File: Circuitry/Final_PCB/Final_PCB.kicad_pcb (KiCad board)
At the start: 2 copper layers, 28 parts

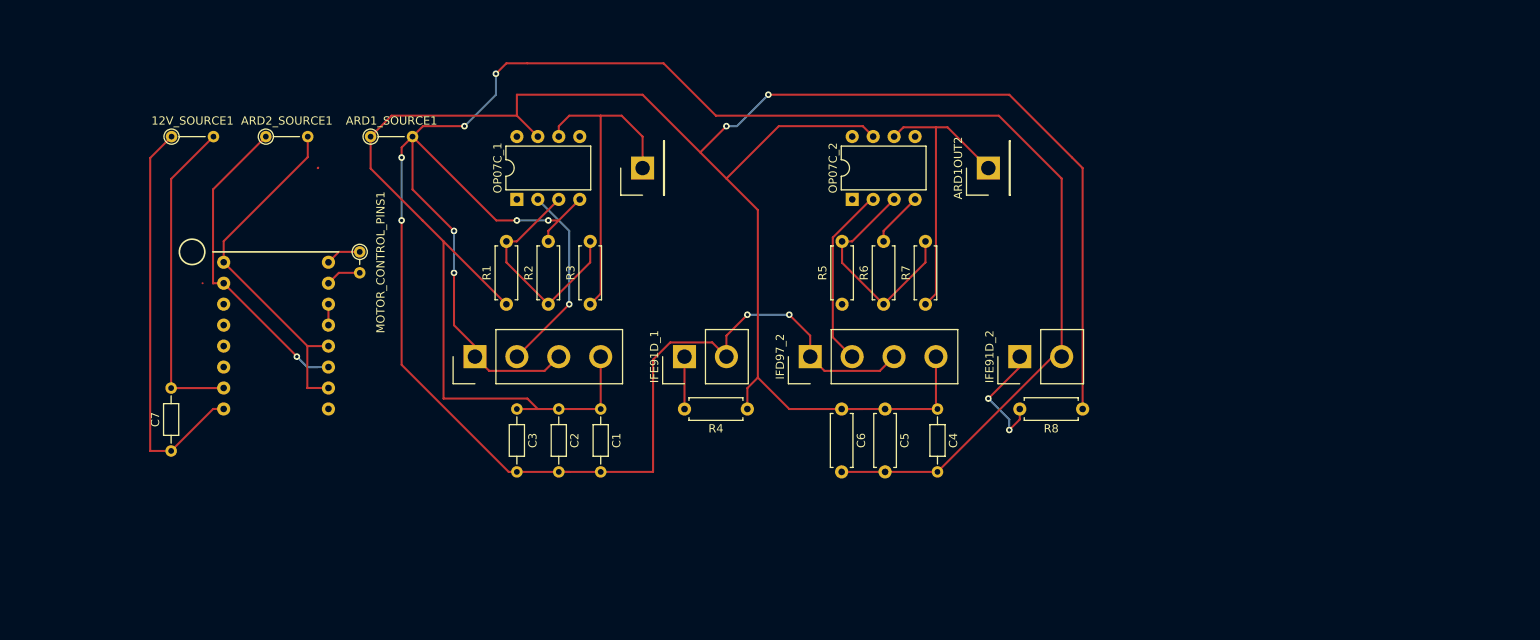
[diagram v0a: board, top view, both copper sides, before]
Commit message: PCB Finalized and updates to python program
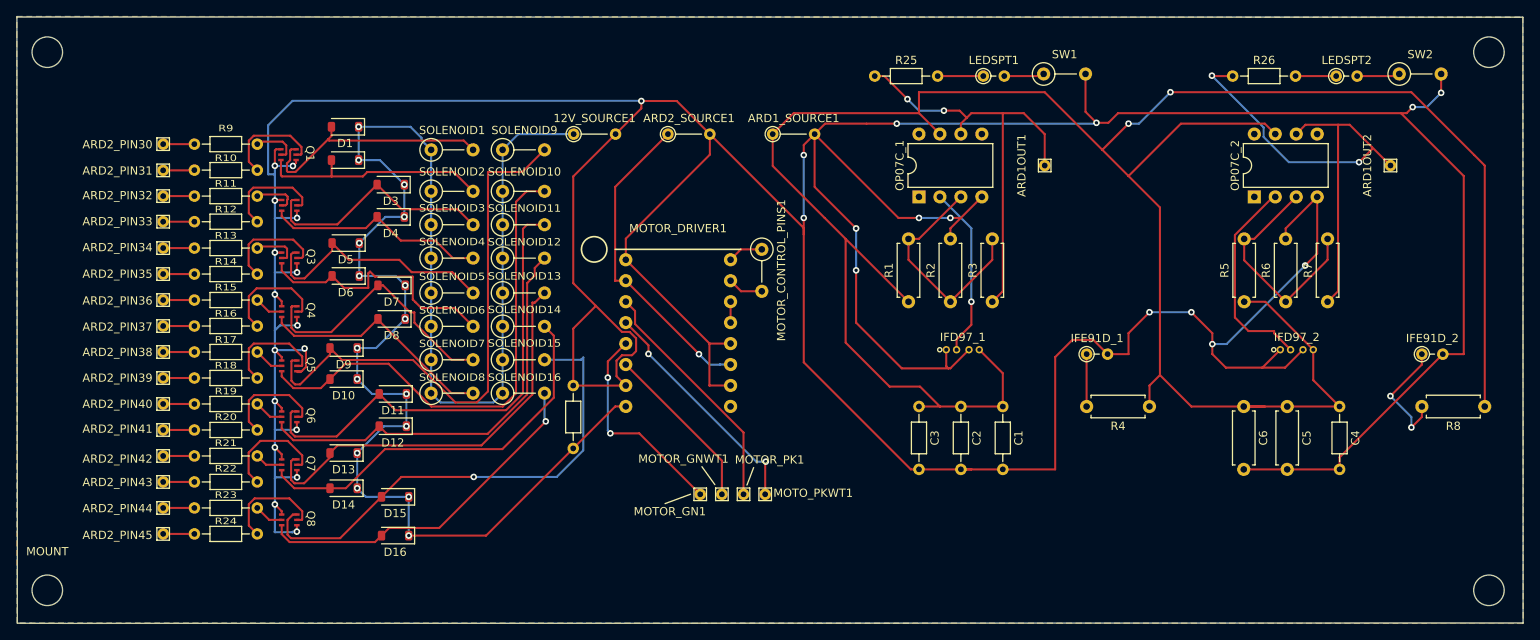
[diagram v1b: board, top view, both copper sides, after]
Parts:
- added ARD2_PIN30: Conn_01x01, Final_PCB_Footprint:ARD_OUT, F.Cu at (95.6, 82.2)
- added ARD2_PIN31: Conn_01x01, Final_PCB_Footprint:ARD_OUT, F.Cu at (95.6, 85.4)
- added ARD2_PIN32: Conn_01x01, Final_PCB_Footprint:ARD_OUT, F.Cu at (95.6, 88.5)
- added ARD2_PIN33: Conn_01x01, Final_PCB_Footprint:ARD_OUT, F.Cu at (95.6, 91.6)
- added ARD2_PIN34: Conn_01x01, Final_PCB_Footprint:ARD_OUT, F.Cu at (95.6, 94.8)
- added ARD2_PIN35: Conn_01x01, Final_PCB_Footprint:ARD_OUT, F.Cu at (95.6, 97.9)
- added ARD2_PIN36: Conn_01x01, Final_PCB_Footprint:ARD_OUT, F.Cu at (95.6, 101.1)
- added ARD2_PIN37: Conn_01x01, Final_PCB_Footprint:ARD_OUT, F.Cu at (95.6, 104.2)
- added ARD2_PIN38: Conn_01x01, Final_PCB_Footprint:ARD_OUT, F.Cu at (95.6, 107.4)
- added ARD2_PIN39: Conn_01x01, Final_PCB_Footprint:ARD_OUT, F.Cu at (95.6, 110.5)
- added ARD2_PIN40: Conn_01x01, Final_PCB_Footprint:ARD_OUT, F.Cu at (95.6, 113.7)
- added ARD2_PIN41: Conn_01x01, Final_PCB_Footprint:ARD_OUT, F.Cu at (95.6, 116.8)
- added ARD2_PIN42: Conn_01x01, Final_PCB_Footprint:ARD_OUT, F.Cu at (95.6, 120.0)
- added ARD2_PIN43: Conn_01x01, Final_PCB_Footprint:ARD_OUT, F.Cu at (95.6, 123.1)
- added ARD2_PIN44: Conn_01x01, Final_PCB_Footprint:ARD_OUT, F.Cu at (95.6, 126.3)
- added ARD2_PIN45: Conn_01x01, Final_PCB_Footprint:ARD_OUT, F.Cu at (95.6, 129.4)
- added D1: MBR0540, Diode_SMD:D_SOD-123, F.Cu at (117.6, 80.1)
- added D10: MBR0540, Diode_SMD:D_SOD-123, F.Cu at (117.4, 110.7)
- added D11: MBR0540, Diode_SMD:D_SOD-123, F.Cu at (123.4, 112.5)
- added D12: MBR0540, Diode_SMD:D_SOD-123, F.Cu at (123.4, 116.4)
- added D13: MBR0540, Diode_SMD:D_SOD-123, F.Cu at (117.4, 119.6)
- added D14: MBR0540, Diode_SMD:D_SOD-123, F.Cu at (117.4, 123.9)
- added D15: MBR0540, Diode_SMD:D_SOD-123, F.Cu at (123.7, 124.9)
- added D16: MBR0540, Diode_SMD:D_SOD-123, F.Cu at (123.7, 129.6)
- added D2: MBR0540, Diode_SMD:D_SOD-123, F.Cu at (117.6, 84.1)
- added D3: MBR0540, Diode_SMD:D_SOD-123, F.Cu at (123.1, 87.1)
- added D4: MBR0540, Diode_SMD:D_SOD-123, F.Cu at (123.1, 91.0)
- added D5: MBR0540, Diode_SMD:D_SOD-123, F.Cu at (117.7, 94.2)
- added D6: MBR0540, Diode_SMD:D_SOD-123, F.Cu at (117.7, 98.2)
- added D7: MBR0540, Diode_SMD:D_SOD-123, F.Cu at (123.2, 99.3)
- added D8: MBR0540, Diode_SMD:D_SOD-123, F.Cu at (123.2, 103.4)
- added D9: MBR0540, Diode_SMD:D_SOD-123, F.Cu at (117.4, 106.9)
- added LEDSPT1: Conn_01x02, Resistor_THT:R_Axial_DIN0204_L3.6mm_D1.6mm_P2.54mm_Vertical, F.Cu at (195.0, 73.9)
- added LEDSPT2: Conn_01x02, Resistor_THT:R_Axial_DIN0204_L3.6mm_D1.6mm_P2.54mm_Vertical, F.Cu at (237.7, 73.9)
- added MOTOR_GN1: Conn_01x01, Final_PCB_Footprint:ARD_OUT, F.Cu at (160.7, 124.6)
- added MOTOR_GNWT1: Conn_01x01, Final_PCB_Footprint:ARD_OUT, F.Cu at (163.3, 124.6)
- added MOTOR_PK1: Conn_01x01, Final_PCB_Footprint:ARD_OUT, F.Cu at (165.9, 124.6)
- added MOTO_PKWT1: Conn_01x01, Final_PCB_Footprint:ARD_OUT, F.Cu at (168.5, 124.6)
- added MOUNT: MountingHole_3.7mm, MountingHole:MountingHole_3.7mm, F.Cu at (81.5, 136.3)
- added Q1: Q_Dual_NMOS_S1G1D2S2G2D1, Final_PCB_Footprint:TSOP6_MOSFET, F.Cu at (110.7, 83.5)
- added Q2: Q_Dual_NMOS_S1G1D2S2G2D1, Final_PCB_Footprint:TSOP6_MOSFET, F.Cu at (110.8, 89.6)
- added Q3: Q_Dual_NMOS_S1G1D2S2G2D1, Final_PCB_Footprint:TSOP6_MOSFET, F.Cu at (110.8, 96.0)
- added Q4: Q_Dual_NMOS_S1G1D2S2G2D1, Final_PCB_Footprint:TSOP6_MOSFET, F.Cu at (110.8, 102.5)
- added Q5: Q_Dual_NMOS_S1G1D2S2G2D1, Final_PCB_Footprint:TSOP6_MOSFET, F.Cu at (110.8, 109.1)
- added Q6: Q_Dual_NMOS_S1G1D2S2G2D1, Final_PCB_Footprint:TSOP6_MOSFET, F.Cu at (110.8, 115.2)
- added Q7: Q_Dual_NMOS_S1G1D2S2G2D1, Final_PCB_Footprint:TSOP6_MOSFET, F.Cu at (110.8, 121.1)
- added Q8: Q_Dual_NMOS_S1G1D2S2G2D1, Final_PCB_Footprint:TSOP6_MOSFET, F.Cu at (110.8, 127.7)
- added R10: R, Resistor_THT:R_Axial_DIN0204_L3.6mm_D1.6mm_P7.62mm_Horizontal, F.Cu at (99.3, 85.3)
- added R11: R, Resistor_THT:R_Axial_DIN0204_L3.6mm_D1.6mm_P7.62mm_Horizontal, F.Cu at (99.3, 88.5)
- added R12: R, Resistor_THT:R_Axial_DIN0204_L3.6mm_D1.6mm_P7.62mm_Horizontal, F.Cu at (99.3, 91.6)
- added R13: R, Resistor_THT:R_Axial_DIN0204_L3.6mm_D1.6mm_P7.62mm_Horizontal, F.Cu at (99.3, 94.8)
- added R14: R, Resistor_THT:R_Axial_DIN0204_L3.6mm_D1.6mm_P7.62mm_Horizontal, F.Cu at (99.3, 97.9)
- added R15: R, Resistor_THT:R_Axial_DIN0204_L3.6mm_D1.6mm_P7.62mm_Horizontal, F.Cu at (99.3, 101.1)
- added R16: R, Resistor_THT:R_Axial_DIN0204_L3.6mm_D1.6mm_P7.62mm_Horizontal, F.Cu at (99.3, 104.2)
- added R17: R, Resistor_THT:R_Axial_DIN0204_L3.6mm_D1.6mm_P7.62mm_Horizontal, F.Cu at (99.3, 107.4)
- added R18: R, Resistor_THT:R_Axial_DIN0204_L3.6mm_D1.6mm_P7.62mm_Horizontal, F.Cu at (99.3, 110.5)
- added R19: R, Resistor_THT:R_Axial_DIN0204_L3.6mm_D1.6mm_P7.62mm_Horizontal, F.Cu at (99.3, 113.7)
- added R20: R, Resistor_THT:R_Axial_DIN0204_L3.6mm_D1.6mm_P7.62mm_Horizontal, F.Cu at (99.3, 116.8)
- added R21: R, Resistor_THT:R_Axial_DIN0204_L3.6mm_D1.6mm_P7.62mm_Horizontal, F.Cu at (99.3, 120.0)
- added R22: R, Resistor_THT:R_Axial_DIN0204_L3.6mm_D1.6mm_P7.62mm_Horizontal, F.Cu at (99.3, 123.1)
- added R23: R, Resistor_THT:R_Axial_DIN0204_L3.6mm_D1.6mm_P7.62mm_Horizontal, F.Cu at (99.3, 126.3)
- added R24: R, Resistor_THT:R_Axial_DIN0204_L3.6mm_D1.6mm_P7.62mm_Horizontal, F.Cu at (99.3, 129.4)
- added R25: R, Resistor_THT:R_Axial_DIN0204_L3.6mm_D1.6mm_P7.62mm_Horizontal, F.Cu at (181.8, 73.9)
- added R26: R, Resistor_THT:R_Axial_DIN0204_L3.6mm_D1.6mm_P7.62mm_Horizontal, F.Cu at (225.2, 73.9)
- added R9: R, Resistor_THT:R_Axial_DIN0204_L3.6mm_D1.6mm_P7.62mm_Horizontal, F.Cu at (99.3, 82.2)
- added REF**: MountingHole_3.7mm, MountingHole:MountingHole_3.7mm, F.Cu at (81.5, 71.0)
- added REF**: MountingHole_3.7mm, MountingHole:MountingHole_3.7mm, F.Cu at (256.3, 71.0)
- added REF**: MountingHole_3.7mm, MountingHole:MountingHole_3.7mm, F.Cu at (256.3, 136.3)
- added SOLENOID1: Conn_01x02, Resistor_THT:R_Axial_DIN0207_L6.3mm_D2.5mm_P5.08mm_Vertical, F.Cu at (128.0, 82.9)
- added SOLENOID10: Conn_01x02, Resistor_THT:R_Axial_DIN0207_L6.3mm_D2.5mm_P5.08mm_Vertical, F.Cu at (136.7, 87.9)
- added SOLENOID11: Conn_01x02, Resistor_THT:R_Axial_DIN0207_L6.3mm_D2.5mm_P5.08mm_Vertical, F.Cu at (136.7, 92.0)
- added SOLENOID12: Conn_01x02, Resistor_THT:R_Axial_DIN0207_L6.3mm_D2.5mm_P5.08mm_Vertical, F.Cu at (136.7, 96.0)
- added SOLENOID13: Conn_01x02, Resistor_THT:R_Axial_DIN0207_L6.3mm_D2.5mm_P5.08mm_Vertical, F.Cu at (136.7, 100.2)
- added SOLENOID14: Conn_01x02, Resistor_THT:R_Axial_DIN0207_L6.3mm_D2.5mm_P5.08mm_Vertical, F.Cu at (136.7, 104.3)
- added SOLENOID15: Conn_01x02, Resistor_THT:R_Axial_DIN0207_L6.3mm_D2.5mm_P5.08mm_Vertical, F.Cu at (136.7, 108.3)
- added SOLENOID16: Conn_01x02, Resistor_THT:R_Axial_DIN0207_L6.3mm_D2.5mm_P5.08mm_Vertical, F.Cu at (136.7, 112.4)
- added SOLENOID2: Conn_01x02, Resistor_THT:R_Axial_DIN0207_L6.3mm_D2.5mm_P5.08mm_Vertical, F.Cu at (128.0, 87.9)
- added SOLENOID3: Conn_01x02, Resistor_THT:R_Axial_DIN0207_L6.3mm_D2.5mm_P5.08mm_Vertical, F.Cu at (128.0, 92.0)
- added SOLENOID4: Conn_01x02, Resistor_THT:R_Axial_DIN0207_L6.3mm_D2.5mm_P5.08mm_Vertical, F.Cu at (128.0, 96.0)
- added SOLENOID5: Conn_01x02, Resistor_THT:R_Axial_DIN0207_L6.3mm_D2.5mm_P5.08mm_Vertical, F.Cu at (128.0, 100.2)
- added SOLENOID6: Conn_01x02, Resistor_THT:R_Axial_DIN0207_L6.3mm_D2.5mm_P5.08mm_Vertical, F.Cu at (128.0, 104.3)
- added SOLENOID7: Conn_01x02, Resistor_THT:R_Axial_DIN0207_L6.3mm_D2.5mm_P5.08mm_Vertical, F.Cu at (128.0, 108.3)
- added SOLENOID8: Conn_01x02, Resistor_THT:R_Axial_DIN0207_L6.3mm_D2.5mm_P5.08mm_Vertical, F.Cu at (128.0, 112.4)
- added SOLENOID9: Conn_01x02, Resistor_THT:R_Axial_DIN0207_L6.3mm_D2.5mm_P5.08mm_Vertical, F.Cu at (136.7, 82.9)
- added SW1: SW_SPST, Resistor_THT:R_Axial_DIN0207_L6.3mm_D2.5mm_P5.08mm_Vertical, F.Cu at (202.3, 73.7)
- added SW2: SW_SPST, Resistor_THT:R_Axial_DIN0207_L6.3mm_D2.5mm_P5.08mm_Vertical, F.Cu at (245.4, 73.7)
- ARD1OUT1, ARD1OUT2: footprint Connector_Samtec_HPM_THT:Samtec_HPM-01-01-x-S_Straight_1x01_Pitch5.08mm -> Final_PCB_Footprint:ARD_OUT
- IFD97_1: footprint Connector_Samtec_HPM_THT:Samtec_HPM-04-05-x-S_Straight_1x04_Pitch5.08mm -> Final_PCB_Footprint:IFD97
- IFD97_2: footprint Connector_Samtec_HPM_THT:Samtec_HPM-04-01-x-S_Straight_1x04_Pitch5.08mm -> Final_PCB_Footprint:IFD97
- IFE91D_1: footprint Connector_Samtec_HPM_THT:Samtec_HPM-02-01-x-S_Straight_1x02_Pitch5.08mm -> Resistor_THT:R_Axial_DIN0204_L3.6mm_D1.6mm_P2.54mm_Vertical
- IFE91D_2: footprint Connector_Samtec_HPM_THT:Samtec_HPM-02-05-x-S_Straight_1x02_Pitch5.08mm -> Resistor_THT:R_Axial_DIN0204_L3.6mm_D1.6mm_P2.54mm_Vertical
- MOTOR_CONTROL_PINS1: footprint Resistor_THT:R_Axial_DIN0204_L3.6mm_D1.6mm_P2.54mm_Vertical -> Resistor_THT:R_Axial_DIN0207_L6.3mm_D2.5mm_P5.08mm_Vertical
- moved IFD97_1 59.1 mm to (192.5, 107.1), turned to 0 degrees
- moved IFD97_2 59.0 mm to (233.0, 107.1), turned to 0 degrees
- moved 12V_SOURCE1 48.7 mm to (145.3, 81.0)
- moved ARD1OUT1 48.7 mm to (202.4, 84.8)
- moved ARD2_SOURCE1 48.7 mm to (156.7, 81.0)
- moved C1 48.7 mm to (197.3, 114.0)
- moved C2 48.7 mm to (192.3, 114.0)
- moved C3 48.7 mm to (187.2, 114.0)
- moved C4 48.7 mm to (238.2, 114.0)
- moved C5 48.7 mm to (231.8, 114.0)
- moved IFE91D_1 48.7 mm to (207.5, 107.6), turned to 0 degrees
- moved IFE91D_2 48.7 mm to (248.1, 107.6), turned to 0 degrees
- moved MOTOR_CONTROL_PINS1 48.7 mm to (168.1, 94.9)
- moved MOTOR_DRIVER1 48.7 mm to (158.0, 105.1)
- moved OP07C_1 48.7 mm to (187.2, 88.6)
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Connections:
- ARD1_SOURCE1 pad 2: /5V_GND_ARD1 -> /12V_GND
- ARD2_SOURCE1 pad 2: /5V_GND_ARD2 -> /12V_GND
- C1 pad 2: /5V_GND_ARD1 -> /12V_GND
- C2 pad 2: /5V_GND_ARD1 -> /12V_GND
- C3 pad 2: /5V_GND_ARD1 -> /12V_GND
- C4 pad 2: /5V_GND_ARD1 -> /12V_GND
- C5 pad 2: /5V_GND_ARD1 -> /12V_GND
- C6 pad 2: /5V_GND_ARD1 -> /12V_GND
- IFD97_1 pad 1: /5V_GND_ARD1 -> /12V_GND
- IFD97_1 pad 3: /5V_GND_ARD1 -> /12V_GND
- IFD97_2 pad 1: /5V_GND_ARD1 -> /12V_GND
- IFD97_2 pad 3: /5V_GND_ARD1 -> /12V_GND
- IFE91D_1 pad 2: /5V_GND_ARD1 -> /12V_GND
- IFE91D_2 pad 2: /5V_GND_ARD1 -> /12V_GND
- MOTOR_DRIVER1 pad 1: /5V_GND_ARD2 -> /12V_GND
- MOTOR_DRIVER1 pad 10: /5V_GND_ARD2 -> /12V_GND
- MOTOR_DRIVER1 pad 12: /5V_GND_ARD2 -> /12V_GND
- MOTOR_DRIVER1 pad 3: unconnected-(MOTOR_DRIVER1-Pin_3-Pad3) -> /MOTOR_PK
- MOTOR_DRIVER1 pad 4: unconnected-(MOTOR_DRIVER1-Pin_4-Pad4) -> /MOTOR_PKWT
- MOTOR_DRIVER1 pad 5: unconnected-(MOTOR_DRIVER1-Pin_5-Pad5) -> /MOTOR_GN
- MOTOR_DRIVER1 pad 6: unconnected-(MOTOR_DRIVER1-Pin_6-Pad6) -> /MOTOR_GNWT
- OP07C_1 pad 4: /5V_GND_ARD1 -> /12V_GND
- OP07C_2 pad 4: /5V_GND_ARD1 -> /12V_GND
- R2 pad 2: /5V_GND_ARD1 -> /12V_GND
- R6 pad 2: /5V_GND_ARD1 -> /12V_GND
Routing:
- net /12V_GND: track 39.0 -> 653.7 mm, vias 0 -> 31
- net /5V_GND_ARD1: track 338.7 -> 0.00 mm, vias 10 -> 0
- net /+12V: track 50.2 -> 201.1 mm, vias 0 -> 16
- net Net-(D9-A): track 0.00 -> 67.2 mm
- net Net-(D10-A): track 0.00 -> 60.9 mm
- net Net-(D15-A): track 0.00 -> 59.7 mm, vias 0 -> 1
- net Net-(D11-A): track 0.00 -> 58.1 mm
- net Net-(D12-A): track 0.00 -> 51.6 mm
- net Net-(D13-A): track 0.00 -> 50.3 mm
- net Net-(D14-A): track 0.00 -> 47.9 mm
- net /5V_GND_ARD2: track 44.1 -> 0.00 mm
- net Net-(D16-A): track 0.00 -> 43.0 mm, vias 0 -> 1
- net Net-(D7-A): track 0.00 -> 32.3 mm
- net Net-(D6-A): track 0.00 -> 31.8 mm
- net Net-(D5-A): track 0.00 -> 30.3 mm
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- added copper zone on B.Cu, net /12V_GND
- added copper zone on F.Cu, net /12V_GND
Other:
- board outline added: 182.6 x 73.5 mm
